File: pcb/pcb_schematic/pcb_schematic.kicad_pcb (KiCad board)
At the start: 2 copper layers, 35 parts, among them J1 Conn_ST_STDC14, J2 USB_B_Micro, J3 Conn_02x02_Odd_Even, Q1 MMBT3904, Q2 MMBT3904, Q3 MMBT3904, U1 STM32G031K8Tx, U2 MIC5301-3.3YD5, U4 SSD1306 128 x 64 OLED (0x3C), Y1 Crystal

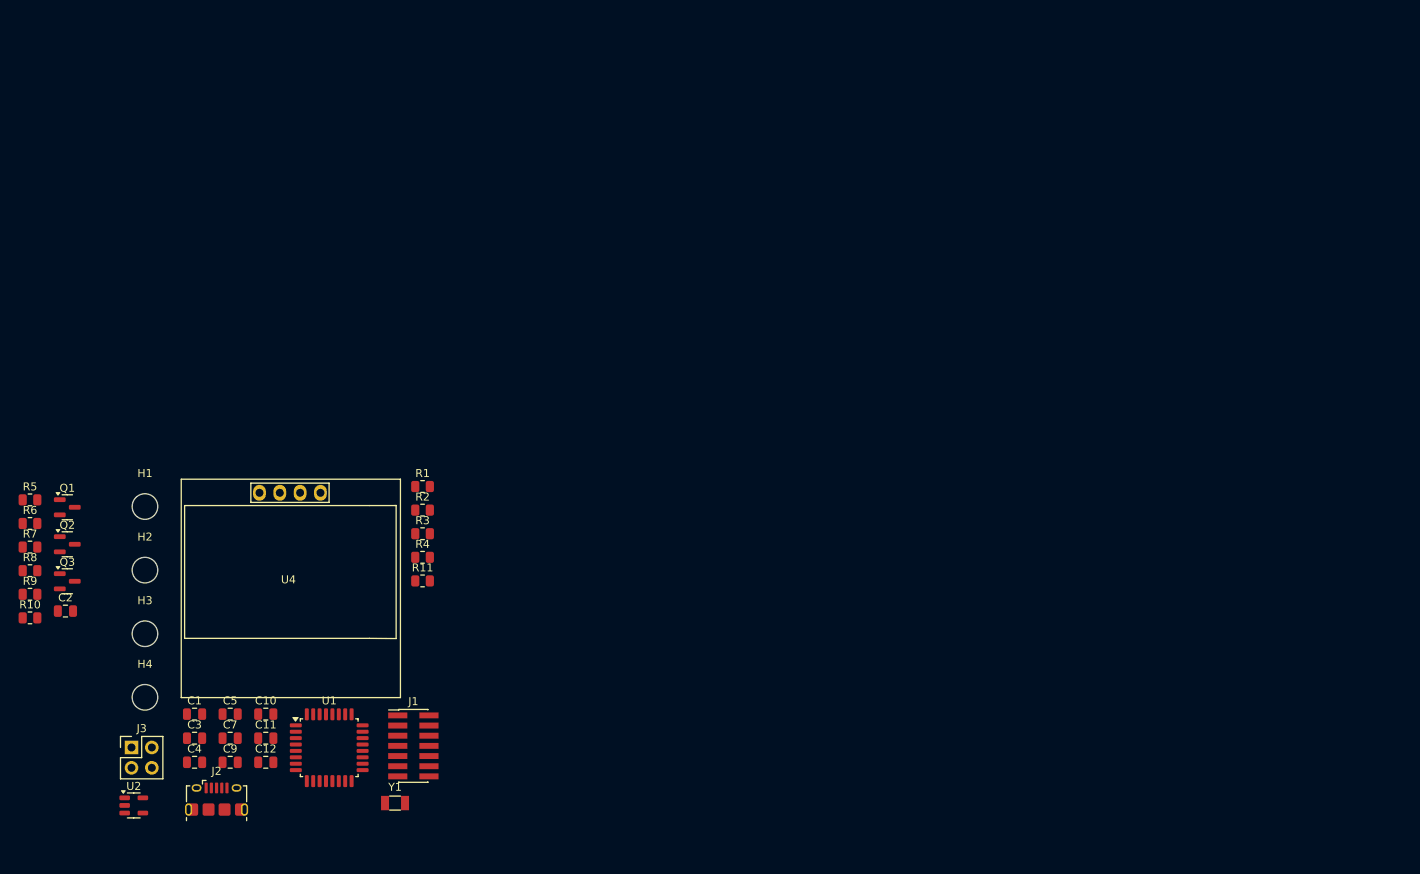
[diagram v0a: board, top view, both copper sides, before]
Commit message: the schmatic keeps chaning i wanna cry
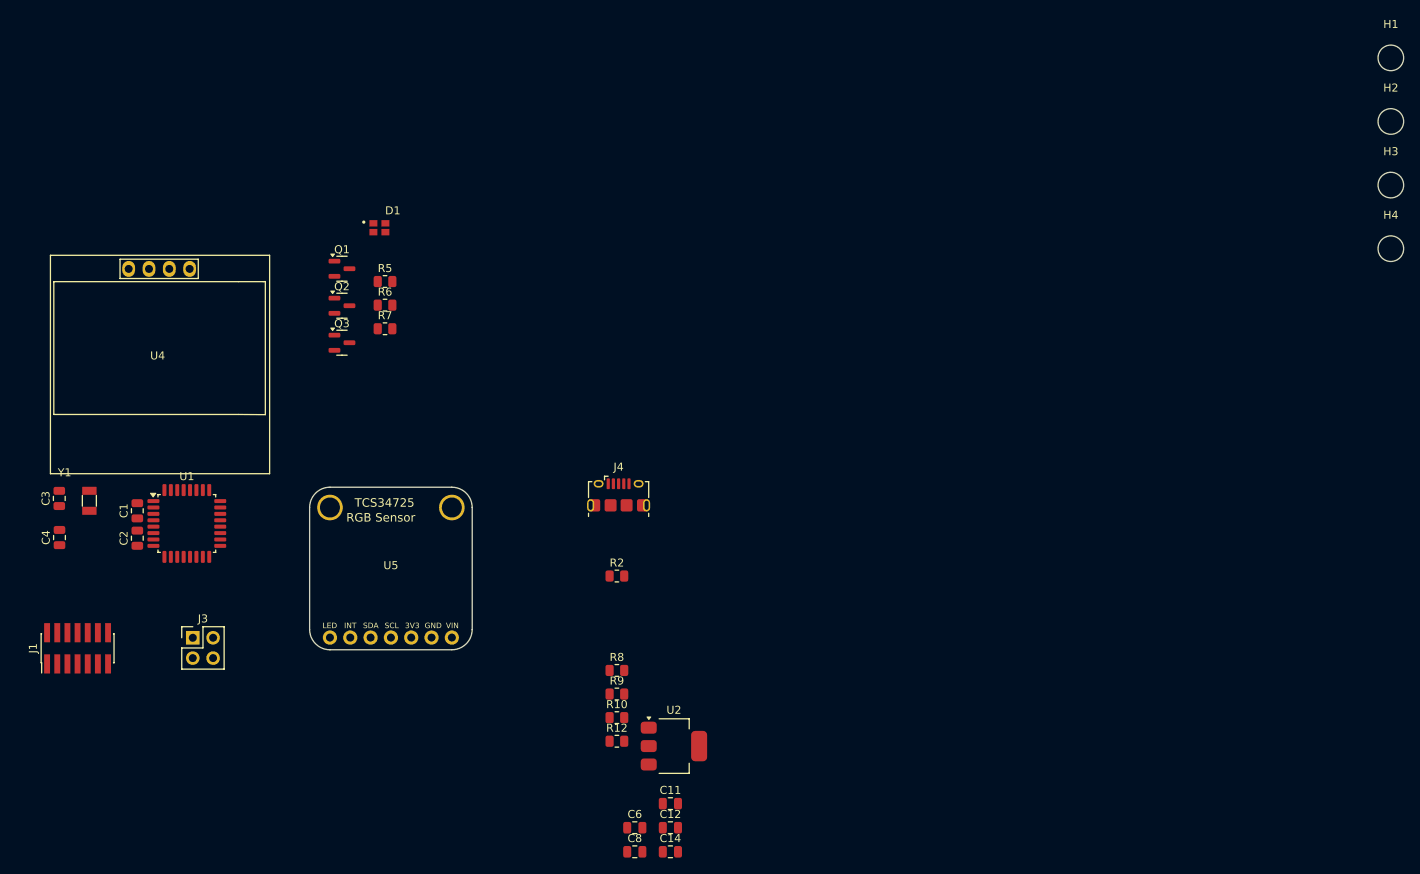
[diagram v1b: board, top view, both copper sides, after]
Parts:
- removed C10, C7: 1uF CER, Capacitor_SMD:C_0805_2012Metric
- removed C5: 4.7nF 1KV, Capacitor_SMD:C_0805_2012Metric
- removed C9: 0.01uF, Capacitor_SMD:C_0805_2012Metric
- removed J2: USB_B_Micro, Connector_USB:USB_Micro-B_Amphenol_10118194_Horizontal
- removed R1: 1M, Resistor_SMD:R_0805_2012Metric
- removed R11: 10K, Resistor_SMD:R_0805_2012Metric
- removed R3: 1.1k, Resistor_SMD:R_0805_2012Metric
- removed R4: 330, Resistor_SMD:R_0805_2012Metric
- added C14: 10uF, Capacitor_SMD:C_0805_2012Metric, F.Cu at (184.7, 119.6)
- added C6: 4.7nF 1KV, Capacitor_SMD:C_0805_2012Metric, F.Cu at (180.2, 116.6)
- added C8: 10uF, Capacitor_SMD:C_0805_2012Metric, F.Cu at (180.2, 119.6)
- added D1: CLMVC-FKA-CLBDGL7LBB79353, RGB_LED:LED_CLMVC-FKA-CLBDGL7LBB79353, F.Cu at (148.3, 41.6)
- added J4: USB_B_Micro, Connector_USB:USB_Micro-B_Amphenol_10118194_Horizontal, F.Cu at (178.2, 75.0)
- added R12: 10K, Resistor_SMD:R_0805_2012Metric, F.Cu at (178.0, 105.8)
- added U5: TCS34725 (0x29), Sensor:TCS34725, F.Cu at (149.8, 73.4)
- R2: value 1k -> 1M
- R5: value 1k -> 470
- R6: value 1.1k -> 220
- R7: value 330 -> 51
- U2: value MIC5301-3.3YD5 -> NCP1117-3.3_SOT223; footprint Package_TO_SOT_SMD:TSOT-23-5 -> Package_TO_SOT_SMD:SOT-223-3_TabPin2
- moved H1 165.5 mm to (274.7, 20.4)
- moved H2 165.5 mm to (274.7, 28.3)
- moved H3 165.5 mm to (274.7, 36.2)
- moved H4 165.5 mm to (274.7, 44.2)
- moved R10 74.4 mm to (178.0, 102.8)
- moved R8 74.4 mm to (178.0, 96.9)
- moved R9 74.4 mm to (178.0, 99.9)
- moved U2 67.9 mm to (185.1, 106.4)
- moved Y1 53.7 mm to (112.0, 75.7), turned to 90 degrees
- moved R5 52.1 mm to (149.0, 48.3)
- moved R6 52.1 mm to (149.0, 51.3)
- moved R7 52.1 mm to (149.0, 54.2)
- moved C11 51.2 mm to (184.7, 113.6)
- moved C12 51.2 mm to (184.7, 116.6)
- moved Q1 45.5 mm to (143.6, 46.7)
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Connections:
- Q2 pad 1: unconnected-(Q2-B-Pad1) -> Net-(Q2-B)
- Q3 pad 1: unconnected-(Q3-B-Pad1) -> Net-(Q3-B)
- R10 pad 2: unconnected-(R10-Pad2) -> Net-(Q3-B)
- R2 pad 1: unconnected-(R2-Pad1) -> Net-(J4-Shield)
- R2 pad 2: unconnected-(R2-Pad2) -> GND
- R9 pad 2: unconnected-(R9-Pad2) -> Net-(Q2-B)
- U1 pad 13: PWM1 -> unconnected-(U1-PA6-Pad13)
- U1 pad 14: PWM2 -> unconnected-(U1-PA7-Pad14)
- U1 pad 18: PWM3 -> PWM1
- U1 pad 22: unconnected-(U1-PA9/PA11-Pad22) -> PWM2
- U1 pad 23: unconnected-(U1-PA10/PA12-Pad23) -> PWM3
- U2 pad 1: VBUS -> GND
- U2 pad 2: GND -> +3.3V
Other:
- board outline added: 20.3 x 20.3 mm
